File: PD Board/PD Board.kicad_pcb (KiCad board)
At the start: 4 copper layers, 80.1 x 46 mm, 19 parts, among them J1 Conn_02x02_Odd_Even, M1 2002411112, P1 2604-1102, P2 2604-1102, P3 2604-1102, P4 2604-1102, P5 2604-1102, P6 2604-1102, P7 2604-1102, P8 2604-1102, U1 MCP1792T-3302H/CB

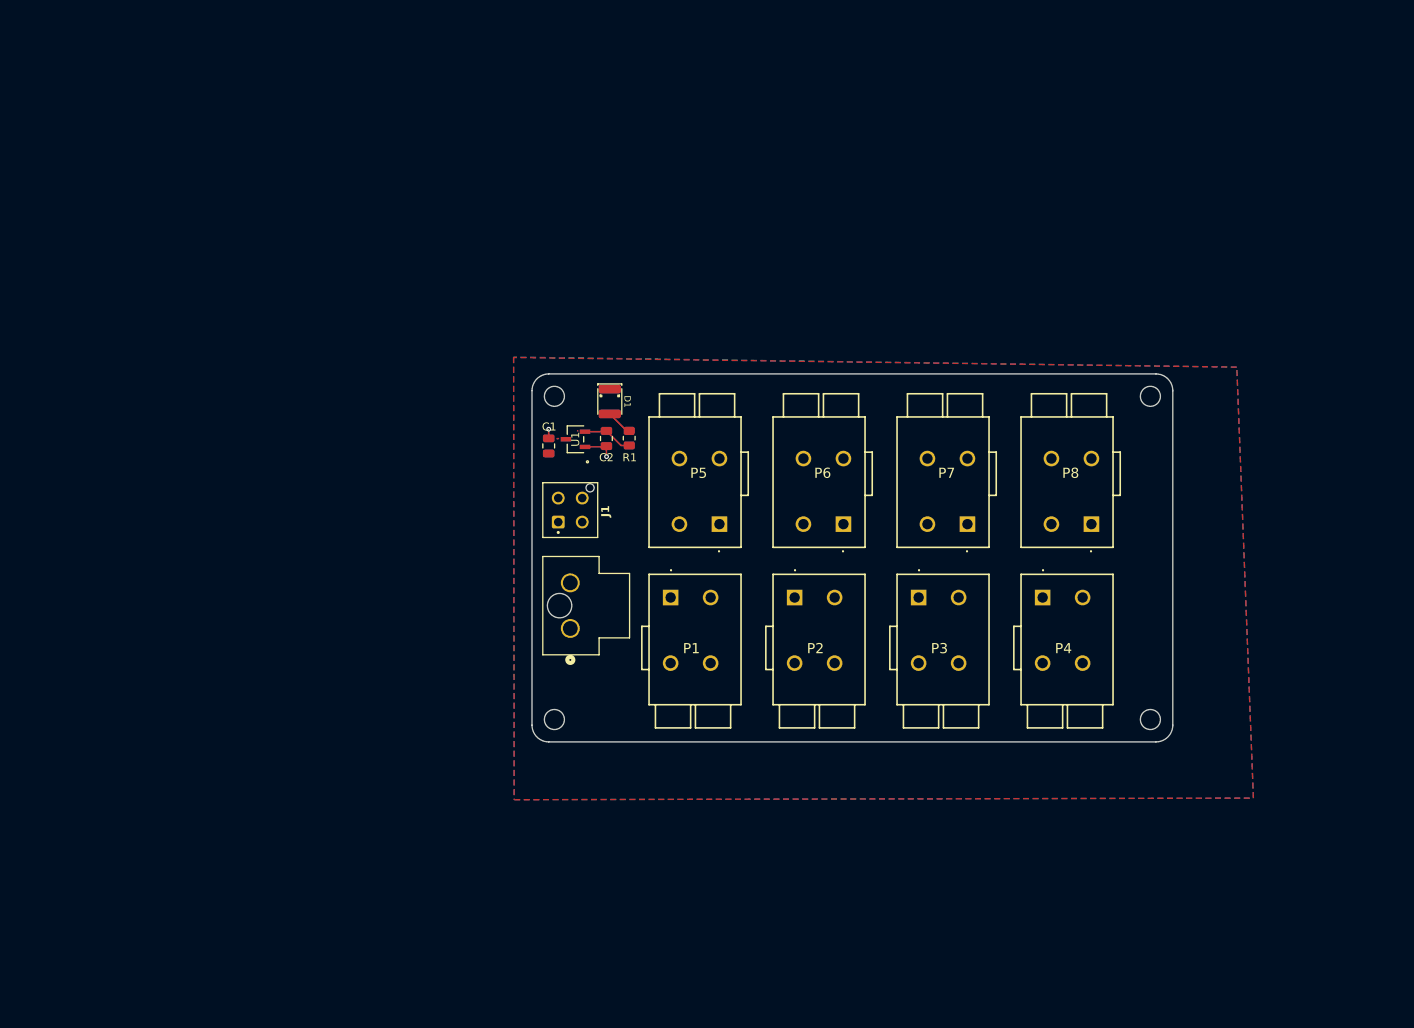
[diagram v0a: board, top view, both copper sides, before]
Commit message: thin pd
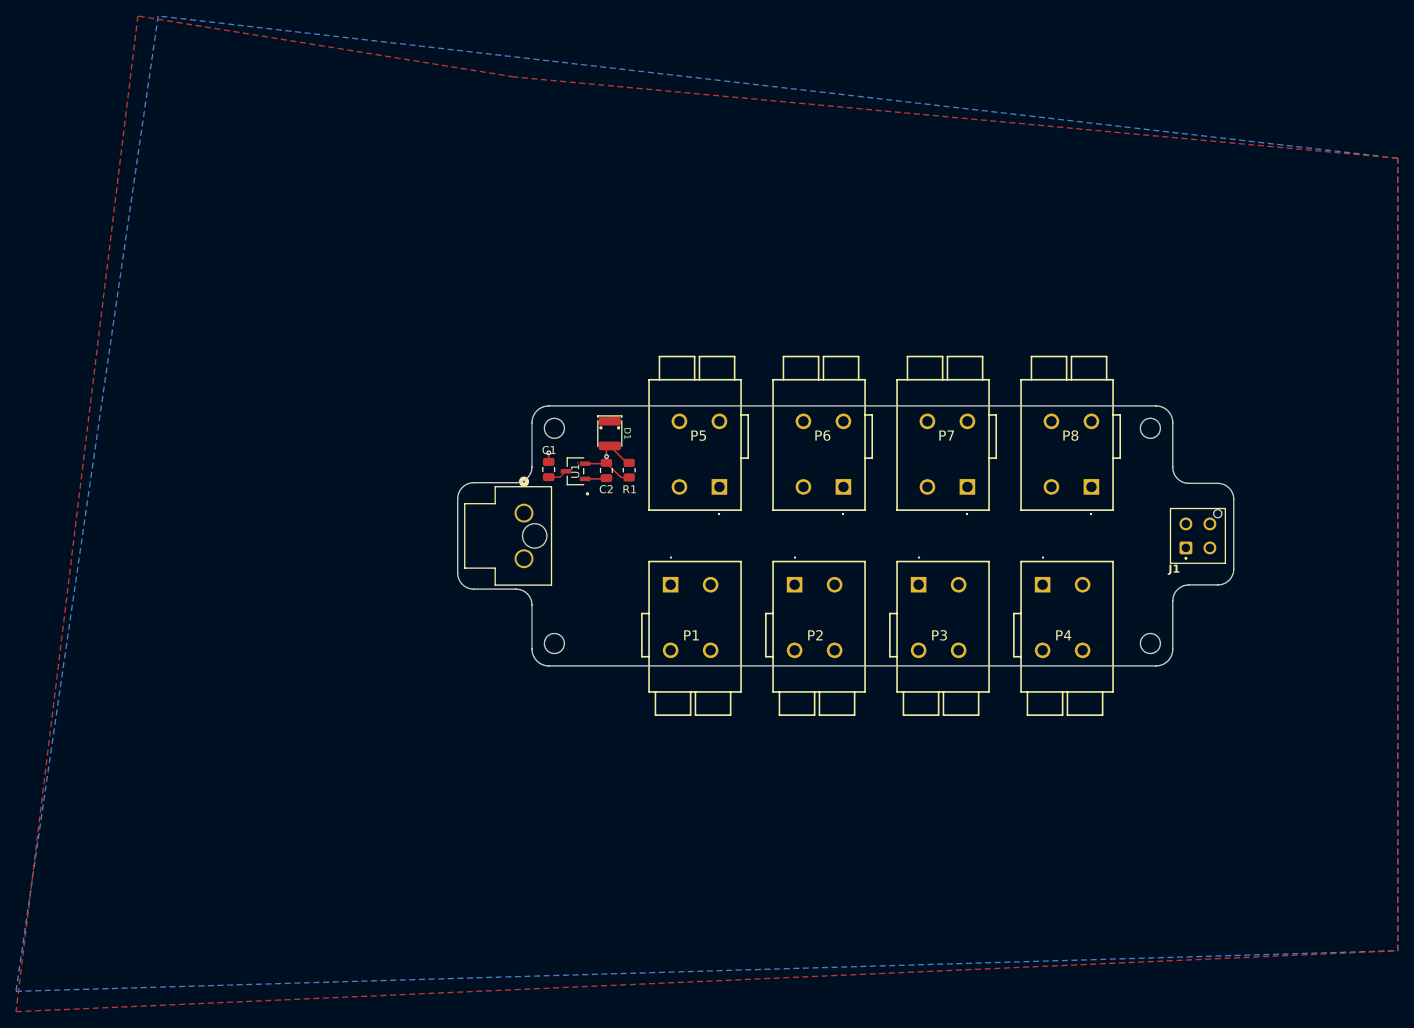
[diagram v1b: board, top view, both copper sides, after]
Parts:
- moved J1 78.5 mm to (171.6, 114.8)
- moved M1 15.5 mm to (88.9, 110.4), turned to 90 degrees
- moved H1 9.50 mm to (92.7, 126.7)
- moved H2 9.50 mm to (167.2, 126.7)
- moved P5 4.65 mm to (113.3, 107.1)
- moved P6 4.65 mm to (128.8, 107.1)
- moved P7 4.65 mm to (144.3, 107.1)
- moved P8 4.65 mm to (159.8, 107.1)
- moved C2 4.00 mm to (99.2, 105.1)
- moved D1 4.00 mm to (99.6, 100.5)
- moved H3 4.00 mm to (167.2, 99.8)
- moved H4 4.00 mm to (92.7, 99.8)
- moved R1 4.00 mm to (102.0, 105.0)
- moved U1 4.00 mm to (95.3, 105.2)
- moved C1 2.95 mm to (92.0, 105.0)
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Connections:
- M1 pad 1: +20V -> GND
- M1 pad 2: GND -> +20V
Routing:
- net +20V: track 0.19 -> 2.45 mm
- added copper zone on In2.Cu, net +20V
- added copper zone on In1.Cu, net GND
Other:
- board size 80.1 x 46 mm -> 97 x 32.5 mm
